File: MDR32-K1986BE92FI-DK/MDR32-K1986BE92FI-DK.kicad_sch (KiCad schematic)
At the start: 57 parts, among them J1 Conn_PROBE, J2 PIN_A, J3 SYS_A, J4 USB_C_Receptacle_USB2.0_16P, J5 PIN_B, J6 SYS_B, Q1 AO3401A, SW1 IT-1181, SW2 SW_DIP_x02, SW3 IT-1181, U1 LM1117GS-3.3, Y1 SMD3225 P4 16MHz, Y2 32.768KHz ±20ppm 6pF

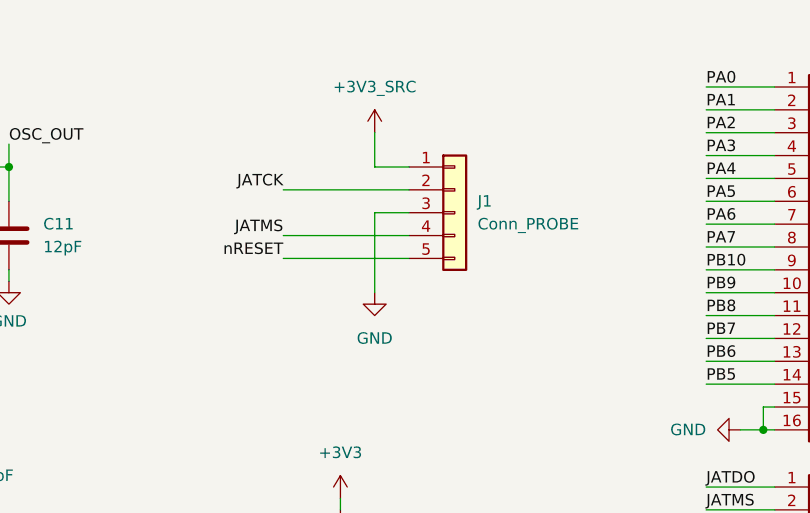
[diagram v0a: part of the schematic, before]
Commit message: fix probe connector
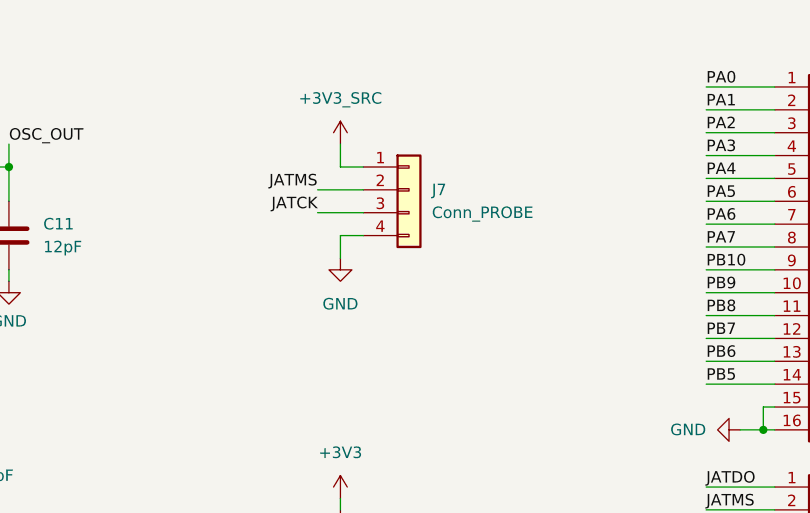
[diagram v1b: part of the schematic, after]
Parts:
- removed J1: Conn_PROBE, Connector_PinHeader_2.54mm:PinHeader_1x05_P2.54mm_Vertical, symbol Connector_Generic:Conn_01x05
- added J7: Conn_PROBE, symbol Connector_Generic:Conn_01x04
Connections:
- net +3V3_SRC: now also J7.1 (Pin_1)
- net GND: now also J7.4 (Pin_4)
- net JATCK: now also J7.3 (Pin_3)
- net JATMS: now also J7.2 (Pin_2)
